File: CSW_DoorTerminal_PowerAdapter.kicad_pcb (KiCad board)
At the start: 2 copper layers, 40 x 30 mm, 4 parts, among them J1 USB_A, J2 S5B-PH-K-S, J3 Screw_Terminal_01x02, J4 Screw_Terminal_01x02

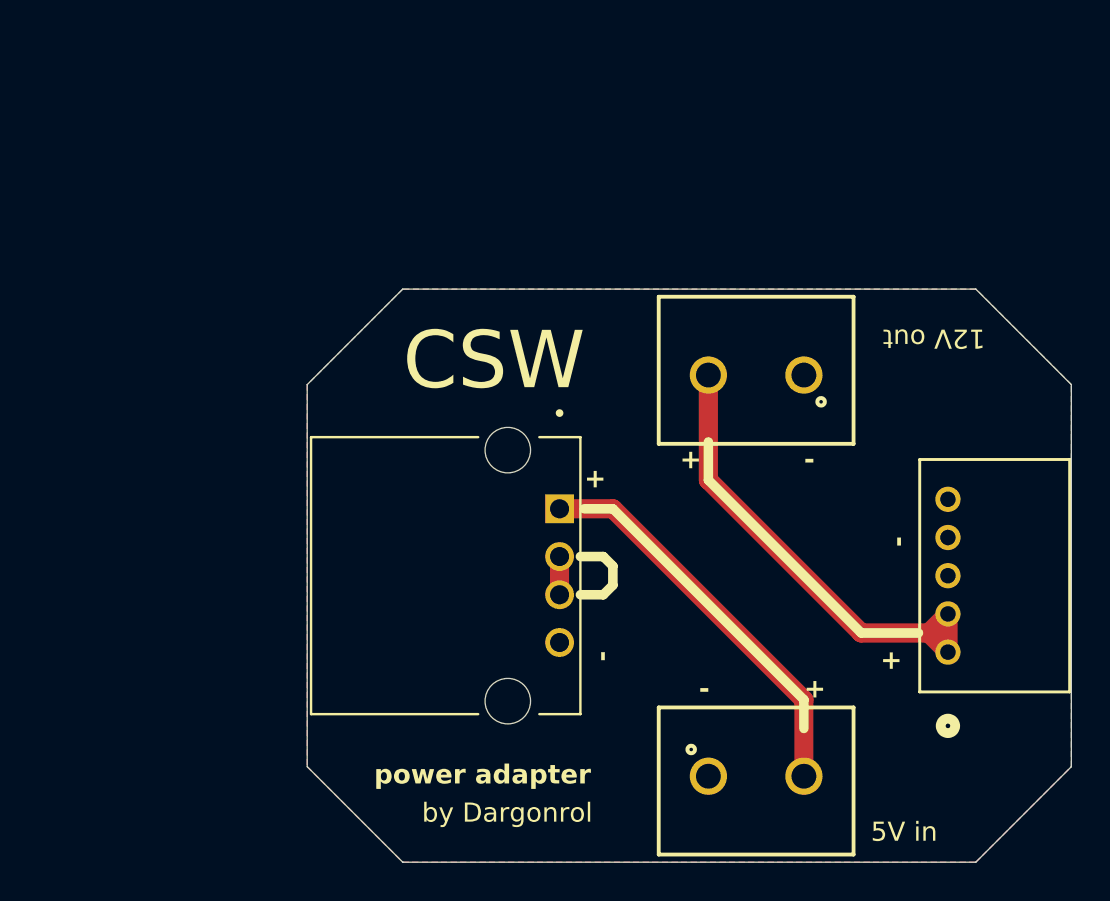
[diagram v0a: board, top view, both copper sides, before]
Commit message: added some metadata
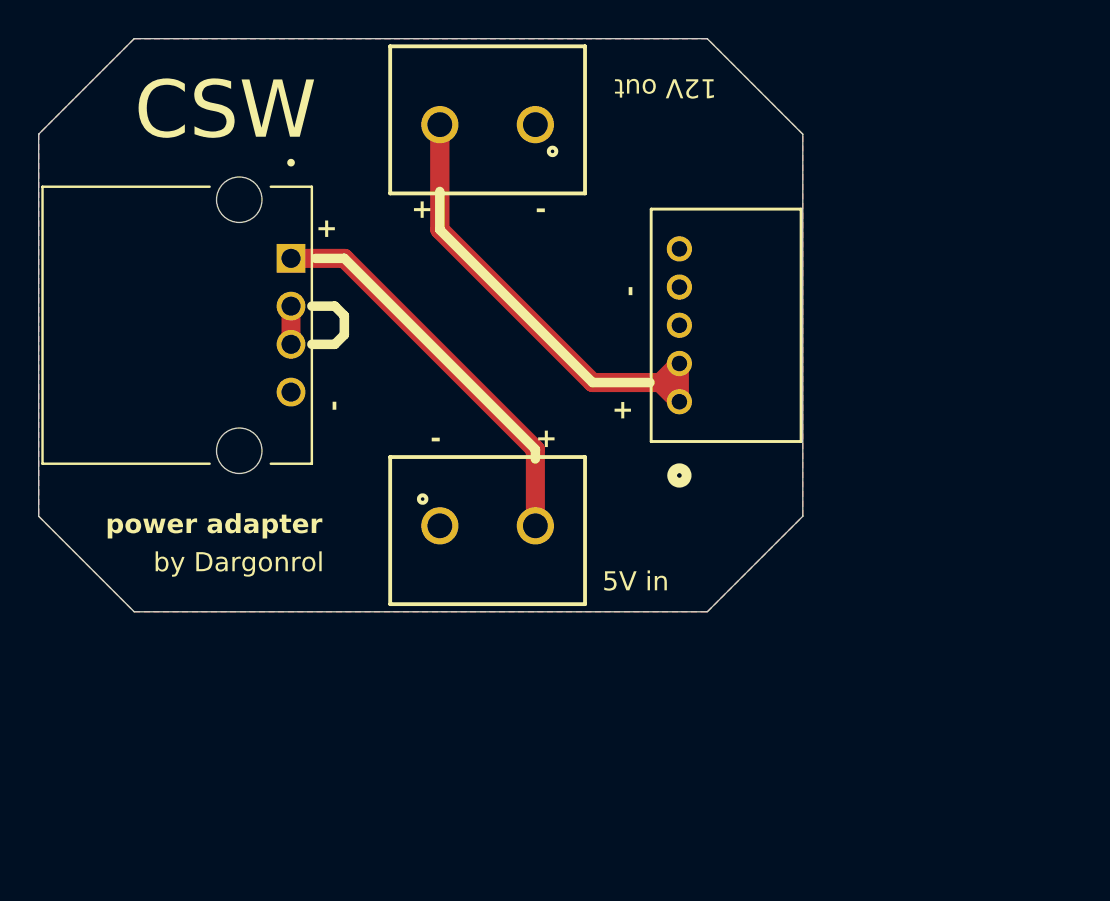
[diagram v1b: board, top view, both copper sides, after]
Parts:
- moved J1 19.2 mm to (96.4, 51.9)
- moved J3 19.2 mm to (109.4, 62.4)
- moved J4 19.2 mm to (109.4, 41.4)
- moved J2 19.2 mm to (119.5, 55.9)
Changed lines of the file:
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@@
 		(legacy_teardrops no)
 	)
-	(paper "A4")
+	(paper "A5")
+	(title_block
+		(title "Door Terminal Adapter PCB")
+		(rev "V1.0")
+	)
 	(layers
 		(0 "F.Cu" signal)
@@
 	(footprint "691137710002:691137710002"
 		(layer "F.Cu")
-		(at 123.5 54.5 180)
+		(at 109.4426 41.3914 180)
 		(property "Reference" "J4"
 			(at -6.5 3 0)
@@
 	(footprint "USB_A1HSW6:OST_USB-A1HSW6"
 		(layer "F.Cu")
-		(at 110.5 65 -90)
+		(at 96.4426 51.8914 -90)
 		(property "Reference" "J1"
 			(at -8.5 9 90)
@@
 		)
 		(property "Value" "USB_A"
-			(at 0.88 -4.96 90)
+			(at 4.5 -4.96 90)
 			(layer "F.Fab")
 			(effects
@@
 	(footprint "S5B-PH-K-S:CONN_S5B-PH-K-S_JST"
 		(layer "F.Cu")
-		(at 133.54 69.0037 90)
+		(at 119.4826 55.8951 90)
 		(tags "S5B-PH-K-S ")
 		(property "Reference" "J2"
@@
 	(footprint "691137710002:691137710002"
 		(layer "F.Cu")
-		(at 123.5 75.5)
+		(at 109.4426 62.3914)
 		(property "Reference" "J3"
 			(at 0 -5.135 0)
@@
 	)
 	(gr_line
-		(start 114.3 64)
-		(end 115.5 64)
+		(start 100.2426 50.8914)
+		(end 101.4426 50.8914)
 		(stroke
 			(width 0.5)
@@
 	)
 	(gr_line
-		(start 114.3 66)
-		(end 115.5 66)
+		(start 100.2426 52.8914)
+		(end 101.4426 52.8914)
 		(stroke
 			(width 0.5)
@@
 	)
 	(gr_line
-		(start 114.5 61.5)
-		(end 116 61.5)
+		(start 100.4426 48.3914)
+		(end 101.9426 48.3914)
 		(stroke
 			(width 0.5)
@@
 	)
 	(gr_line
-		(start 115.5 64)
-		(end 116 64.5)
+		(start 101.4426 50.8914)
+		(end 101.9426 51.3914)
 		(stroke
 			(width 0.5)
@@
 	)
 	(gr_line
-		(start 115.5 66)
-		(end 116 65.5)
+		(start 101.4426 52.8914)
+		(end 101.9426 52.3914)
 		(stroke
 			(width 0.5)
@@
 	)
 	(gr_line
-		(start 116 61.5)
-		(end 116 61.5)
+		(start 101.9426 48.3914)
+		(end 101.9426 48.3914)
 		(stroke
 			(width 0.5)
@@
 	)
 	(gr_line
-		(start 116 61.5)
-		(end 126 71.5)
+		(start 101.9426 48.3914)
+		(end 111.9426 58.3914)
 		(stroke
 			(width 0.5)
@@
 	)
 	(gr_line
-		(start 116 64.5)
-		(end 116 65.5)
+		(start 101.9426 51.3914)
+		(end 101.9426 52.3914)
 		(stroke
 			(width 0.5)
@@
 	)
 	(gr_line
-		(start 121 60)
-		(end 121 58)
+		(start 106.9426 46.8914)
+		(end 106.9426 44.8914)
 		(stroke
 			(width 0.5)
@@
 	)
 	(gr_line
-		(start 126 71.5)
-		(end 126 73)
+		(start 111.9426 58.8914)
+		(end 111.9426 58.3914)
 		(stroke
 			(width 0.5)
@@
 	)
 	(gr_line
-		(start 129 68)
-		(end 121 60)
+		(start 114.9426 54.8914)
+		(end 106.9426 46.8914)
 		(stroke
 			(width 0.5)
@@
 	)
 	(gr_line
-		(start 132 68)
-		(end 129 68)
+		(start 117.9426 54.8914)
+		(end 114.9426 54.8914)
 		(stroke
 			(width 0.5)
@@
 	)
 	(gr_line
-		(start 100 55)
-		(end 100 75)
+		(start 85.9426 41.8914)
+		(end 85.9426 61.8914)
 		(stroke
 			(width 0.05)
@@
 	)
 	(gr_line
-		(start 100 75)
-		(end 105 80)
+		(start 85.9426 61.8914)
+		(end 90.9426 66.8914)
 		(stroke
 			(width 0.05)
@@
 	)
 	(gr_line
-		(start 105 50)
-		(end 100 55)
+		(start 90.9426 36.8914)
+		(end 85.9426 41.8914)
 		(stroke
 			(width 0.05)
@@
 	)
 	(gr_line
-		(start 105 80)
-		(end 135 80)
+		(start 90.9426 66.8914)
+		(end 120.9426 66.8914)
 		(stroke
 			(width 0.05)
@@
 	)
 	(gr_line
-		(start 135 50)
-		(end 105 50)
+		(start 120.9426 36.8914)
+		(end 90.9426 36.8914)
 		(stroke
 			(width 0.05)
@@
 	)
 	(gr_line
-		(start 135 80)
-		(end 140 75)
+		(start 120.9426 66.8914)
+		(end 125.9426 61.8914)
 		(stroke
 			(width 0.05)
@@
 	)
 	(gr_line
-		(start 140 55)
-		(end 135 50)
+		(start 125.9426 41.8914)
+		(end 120.9426 36.8914)
 		(stroke
 			(width 0.05)
@@
 	)
 	(gr_line
-		(start 140 75)
-		(end 140 55)
+		(start 125.9426 61.8914)
+		(end 125.9426 41.8914)
 		(stroke
 			(width 0.05)
@@
 	)
 	(gr_text "by Dargonrol"
-		(at 106 78 0)
+		(at 91.9426 64.8914 0)
 		(layer "F.SilkS")
 		(effects
@@
 	)
 	(gr_text "5V in"
-		(at 129.5 79 0)
+		(at 115.4426 65.8914 0)
 		(layer "F.SilkS")
 		(effects
@@
 	)
 	(gr_text "12V out"
-		(at 135.5 52 180)
+		(at 121.4426 38.8914 180)
 		(layer "F.SilkS")
 		(effects
@@
 	)
 	(gr_text "+"
-		(at 114.5 60.5 0)
+		(at 100.4426 47.3914 0)
 		(layer "F.SilkS")
 		(effects
@@
 	)
 	(gr_text "+"
-		(at 119.5 59.5 0)
+		(at 105.4426 46.3914 0)
 		(layer "F.SilkS")
 		(effects
@@
 	)
 	(gr_text "-"
-		(at 120.5 71.5 0)
+		(at 106.4426 58.3914 0)
 		(layer "F.SilkS")
 		(effects
@@
 	)
 	(gr_text "-"
-		(at 126 59.5 0)
+		(at 111.9426 46.3914 0)
 		(layer "F.SilkS")
 		(effects
@@
 	)
 	(gr_text "+"
-		(at 126 71.5 0)
+		(at 111.9426 58.3914 0)
 		(layer "F.SilkS")
 		(effects
@@
 	)
 	(gr_text "+"
-		(at 130 70 0)
+		(at 115.9426 56.8914 0)
 		(layer "F.SilkS")
 		(effects
@@
 	)
 	(gr_text "-"
-		(at 116 69.5 90)
+		(at 101.9426 56.3914 90)
 		(layer "F.SilkS")
 		(effects
@@
 	)
 	(gr_text "-"
-		(at 131.5 63.5 90)
+		(at 117.4426 50.3914 90)
 		(layer "F.SilkS")
 		(effects
@@
 	)
 	(gr_text "power adapter"
-		(at 103.5 76 0)
+		(at 89.4426 62.8914 0)
 		(layer "F.SilkS")
 		(effects
@@
 	)
 	(gr_text "CSW"
-		(at 105 55.5 0)
+		(at 90.9426 42.3914 0)
 		(layer "F.SilkS")
 		(effects
@@
 	)
 	(segment
-		(start 126 75.5)
-		(end 126 71.5)
+		(start 106.9426 46.8914)
+		(end 114.9426 54.8914)
+		(width 1)
+		(layer "F.Cu")
+		(net "/Vee")
+	)
+	(segment
+		(start 114.9426 54.8914)
+		(end 118.486301 54.8914)
+		(width 1)
+		(layer "F.Cu")
+		(net "/Vee")
+	)
+	(segment
+		(start 106.9426 41.3914)
+		(end 106.9426 46.8914)
+		(width 1)
+		(layer "F.Cu")
+		(net "/Vee")
+	)
+	(segment
+		(start 118.486301 54.8914)
+		(end 119.4826 53.895101)
+		(width 1)
+		(layer "F.Cu")
+		(net "/Vee")
+	)
+	(segment
+		(start 119.4826 55.8951)
+		(end 119.4826 53.895101)
+		(width 1)
+		(layer "F.Cu")
+		(net "/Vee")
+	)
+	(segment
+		(start 119.4826 55.8951)
+		(end 118.486301 54.898801)
+		(width 1)
+		(layer "F.Cu")
+		(net "/Vee")
+	)
+	(segment
+		(start 118.486301 54.898801)
+		(end 118.486301 54.8914)
+		(width 1)
+		(layer "F.Cu")
+		(net "/Vee")
+	)
+	(segment
+		(start 111.9426 62.3914)
+		(end 111.9426 58.3914)
 		(width 1)
 		(layer "F.Cu")
@@
 	)
 	(segment
-		(start 126 71.5)
-		(end 116 61.5)
+		(start 111.9426 58.3914)
+		(end 101.9426 48.3914)
 		(width 1)
 		(layer "F.Cu")
@@
 	)
 	(segment
-		(start 116 61.5)
-		(end 113.21 61.5)
+		(start 101.9426 48.3914)
+		(end 99.1526 48.3914)
 		(width 1)
 		(layer "F.Cu")
@@
 	)
 	(segment
-		(start 113.21 66)
-		(end 113.21 64)
+		(start 99.1526 52.8914)
+		(end 99.1526 50.8914)
 		(width 1)
 		(layer "F.Cu")
 		(net "Net-(J1-D+)")
-	)
-	(segment
-		(start 121 60)
-		(end 129 68)
-		(width 1)
-		(layer "F.Cu")
-		(net "/Vee")
-	)
-	(segment
-		(start 129 68)
-		(end 132.543701 68)
-		(width 1)
-		(layer "F.Cu")
-		(net "/Vee")
-	)
-	(segment
-		(start 121 54.5)
-		(end 121 60)
-		(width 1)
-		(layer "F.Cu")
-		(net "/Vee")
-	)
-	(segment
-		(start 132.543701 68)
-		(end 133.54 67.003701)
-		(width 1)
-		(layer "F.Cu")
-		(net "/Vee")
-	)
-	(segment
-		(start 133.54 69.0037)
-		(end 133.54 67.003701)
-		(width 1)
-		(layer "F.Cu")
-		(net "/Vee")
-	)
-	(segment
-		(start 133.54 69.0037)
-		(end 132.543701 68.007401)
-		(width 1)
-		(layer "F.Cu")
-		(net "/Vee")
-	)
-	(segment
-		(start 132.543701 68.007401)
-		(end 132.543701 68)
-		(width 1)
-		(layer "F.Cu")
-		(net "/Vee")
 	)
 	(zone
@@
 		(polygon
 			(pts
-				(xy 135 50) (xy 105 50) (xy 100 55) (xy 100 75) (xy 105 80) (xy 135 80) (xy 140 75) (xy 140 55)
-			)
-		)
+				(xy 120.9426 36.8914) (xy 90.9426 36.8914) (xy 85.9426 41.8914) (xy 85.9426 61.8914) (xy 90.9426 66.8914)
+				(xy 120.9426 66.8914) (xy 125.9426 61.8914) (xy 125.9426 41.8914)
+			)
+		)
